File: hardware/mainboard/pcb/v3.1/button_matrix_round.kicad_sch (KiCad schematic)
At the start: 6 parts, among them U27 touch_but_round, U28 touch_but_round, U29 touch_but_round

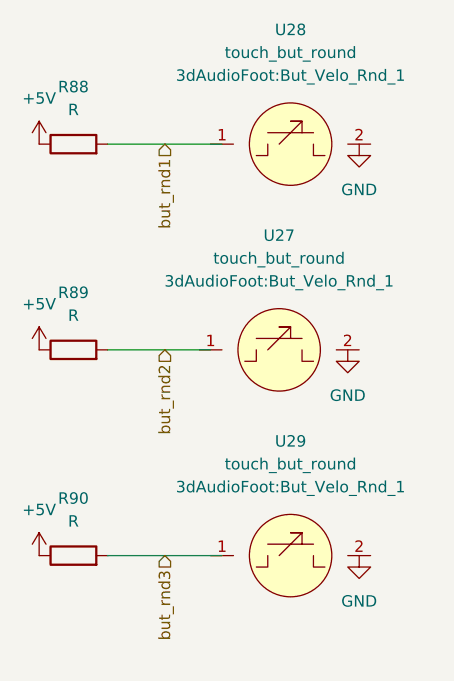
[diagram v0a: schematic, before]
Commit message: .
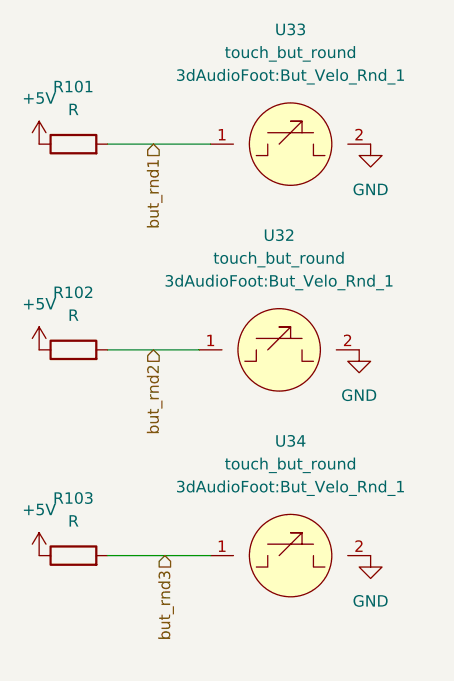
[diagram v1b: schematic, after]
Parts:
- renumbered R88 to R101, R89 to R102, R90 to R103, U27 to U32, U28 to U33, U29 to U34
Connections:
- net GND: now also U32.2, U33.2, U34.2
- net but_rnd1: now also U33.1
- net but_rnd2: now also U32.1
- net but_rnd3: now also U34.1
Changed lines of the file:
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@@
 (kicad_sch (version 20211123) (generator eeschema)
   (paper "A4")
-  (wire (pts (xy 85.09 54.61) (xy 97.79 54.61))
+  (wire (pts (xy 85.09 54.61) (xy 96.52 54.61))
     (stroke (width 0) (type default) (color 0 0 0 0))
   )
-  (wire (pts (xy 85.09 77.47) (xy 96.52 77.47))
+  (wire (pts (xy 85.09 100.33) (xy 96.52 100.33))
     (stroke (width 0) (type default) (color 0 0 0 0))
   )
-  (wire (pts (xy 85.09 100.33) (xy 97.79 100.33))
+  (wire (pts (xy 85.09 77.47) (xy 95.25 77.47))
     (stroke (width 0) (type default) (color 0 0 0 0))
   )
@@
     (effects (font (size 1.27 1.27)) (justify right))
   )
-  (hierarchical_label "but_rnd2" (shape input) (at 91.44 77.47 270)
+  (hierarchical_label "but_rnd2" (shape input) (at 90.17 77.47 270)
     (effects (font (size 1.27 1.27)) (justify right))
   )
-  (hierarchical_label "but_rnd1" (shape input) (at 91.44 54.61 270)
+  (hierarchical_label "but_rnd1" (shape input) (at 90.17 54.61 270)
     (effects (font (size 1.27 1.27)) (justify right))
   )
   (symbol (lib_id "Device:R") (at 81.28 100.33 90) (unit 1)
     (in_bom yes) (on_board yes) (fields_autoplaced)
-    (property "Reference" "R90" (id 0) (at 81.28 93.98 90))
+    (property "Reference" "R103" (id 0) (at 81.28 93.98 90))
     (property "Value" "R" (id 1) (at 81.28 96.52 90))
     (property "Footprint" "Resistor_SMD:R_1206_3216Metric_Pad1.30x1.75mm_HandSolder" (id 2) (at 81.28 102.108 90)
@@
   (symbol (lib_id "Device:R") (at 81.28 54.61 90) (unit 1)
     (in_bom yes) (on_board yes) (fields_autoplaced)
-    (property "Reference" "R88" (id 0) (at 81.28 48.26 90))
+    (property "Reference" "R101" (id 0) (at 81.28 48.26 90))
     (property "Value" "R" (id 1) (at 81.28 50.8 90))
     (property "Footprint" "Resistor_SMD:R_1206_3216Metric_Pad1.30x1.75mm_HandSolder" (id 2) (at 81.28 56.388 90)
@@
     (pin "2")
   )
-  (symbol (lib_id "power:GND") (at 111.76 77.47 0) (unit 1)
+  (symbol (lib_id "power:GND") (at 113.03 77.47 0) (unit 1)
     (in_bom yes) (on_board yes) (fields_autoplaced)
-    (property "Reference" "#PWR070" (id 0) (at 111.76 83.82 0)
+    (property "Reference" "#PWR079" (id 0) (at 113.03 83.82 0)
       (effects (font (size 1.27 1.27)) hide)
     )
-    (property "Value" "GND" (id 1) (at 111.76 82.55 0))
-    (property "Footprint" "" (id 2) (at 111.76 77.47 0)
+    (property "Value" "GND" (id 1) (at 113.03 82.55 0))
+    (property "Footprint" "" (id 2) (at 113.03 77.47 0)
       (effects (font (size 1.27 1.27)) hide)
     )
-    (property "Datasheet" "" (id 3) (at 111.76 77.47 0)
+    (property "Datasheet" "" (id 3) (at 113.03 77.47 0)
       (effects (font (size 1.27 1.27)) hide)
     )
     (pin "1")
   )
-  (symbol (lib_id "power:GND") (at 113.03 100.33 0) (unit 1)
+  (symbol (lib_id "power:GND") (at 114.3 100.33 0) (unit 1)
     (in_bom yes) (on_board yes) (fields_autoplaced)
-    (property "Reference" "#PWR072" (id 0) (at 113.03 106.68 0)
+    (property "Reference" "#PWR081" (id 0) (at 114.3 106.68 0)
       (effects (font (size 1.27 1.27)) hide)
     )
-    (property "Value" "GND" (id 1) (at 113.03 105.41 0))
-    (property "Footprint" "" (id 2) (at 113.03 100.33 0)
+    (property "Value" "GND" (id 1) (at 114.3 105.41 0))
+    (property "Footprint" "" (id 2) (at 114.3 100.33 0)
       (effects (font (size 1.27 1.27)) hide)
     )
-    (property "Datasheet" "" (id 3) (at 113.03 100.33 0)
+    (property "Datasheet" "" (id 3) (at 114.3 100.33 0)
       (effects (font (size 1.27 1.27)) hide)
     )
     (pin "1")
   )
-  (symbol (lib_id "power:GND") (at 113.03 54.61 0) (unit 1)
+  (symbol (lib_id "power:GND") (at 114.3 54.61 0) (unit 1)
     (in_bom yes) (on_board yes) (fields_autoplaced)
-    (property "Reference" "#PWR071" (id 0) (at 113.03 60.96 0)
+    (property "Reference" "#PWR080" (id 0) (at 114.3 60.96 0)
       (effects (font (size 1.27 1.27)) hide)
     )
-    (property "Value" "GND" (id 1) (at 113.03 59.69 0))
-    (property "Footprint" "" (id 2) (at 113.03 54.61 0)
+    (property "Value" "GND" (id 1) (at 114.3 59.69 0))
+    (property "Footprint" "" (id 2) (at 114.3 54.61 0)
       (effects (font (size 1.27 1.27)) hide)
     )
-    (property "Datasheet" "" (id 3) (at 113.03 54.61 0)
+    (property "Datasheet" "" (id 3) (at 114.3 54.61 0)
       (effects (font (size 1.27 1.27)) hide)
     )
@@
   (symbol (lib_id "3dAudioSym:touch_but_round") (at 105.41 101.6 0) (unit 1)
     (in_bom yes) (on_board yes) (fields_autoplaced)
-    (property "Reference" "U29" (id 0) (at 105.41 87.63 0))
+    (property "Reference" "U34" (id 0) (at 105.41 87.63 0))
     (property "Value" "touch_but_round" (id 1) (at 105.41 90.17 0))
     (property "Footprint" "3dAudioFoot:But_Velo_Rnd_1" (id 2) (at 105.41 92.71 0))
@@
   (symbol (lib_id "power:+5V") (at 77.47 100.33 0) (unit 1)
     (in_bom yes) (on_board yes) (fields_autoplaced)
-    (property "Reference" "#PWR069" (id 0) (at 77.47 104.14 0)
+    (property "Reference" "#PWR078" (id 0) (at 77.47 104.14 0)
       (effects (font (size 1.27 1.27)) hide)
     )
@@
   (symbol (lib_id "power:+5V") (at 77.47 77.47 0) (unit 1)
     (in_bom yes) (on_board yes) (fields_autoplaced)
-    (property "Reference" "#PWR068" (id 0) (at 77.47 81.28 0)
+    (property "Reference" "#PWR077" (id 0) (at 77.47 81.28 0)
       (effects (font (size 1.27 1.27)) hide)
     )
@@
   (symbol (lib_name "touch_but_round_1") (lib_id "3dAudioSym:touch_but_round") (at 105.41 55.88 0) (unit 1)
     (in_bom yes) (on_board yes) (fields_autoplaced)
-    (property "Reference" "U28" (id 0) (at 105.41 41.91 0))
+    (property "Reference" "U33" (id 0) (at 105.41 41.91 0))
     (property "Value" "touch_but_round" (id 1) (at 105.41 44.45 0))
     (property "Footprint" "3dAudioFoot:But_Velo_Rnd_1" (id 2) (at 105.41 46.99 0))
@@
   (symbol (lib_id "power:+5V") (at 77.47 54.61 0) (unit 1)
     (in_bom yes) (on_board yes) (fields_autoplaced)
-    (property "Reference" "#PWR067" (id 0) (at 77.47 58.42 0)
+    (property "Reference" "#PWR076" (id 0) (at 77.47 58.42 0)
       (effects (font (size 1.27 1.27)) hide)
     )
@@
   (symbol (lib_id "Device:R") (at 81.28 77.47 90) (unit 1)
     (in_bom yes) (on_board yes) (fields_autoplaced)
-    (property "Reference" "R89" (id 0) (at 81.28 71.12 90))
+    (property "Reference" "R102" (id 0) (at 81.28 71.12 90))
     (property "Value" "R" (id 1) (at 81.28 73.66 90))
     (property "Footprint" "Resistor_SMD:R_1206_3216Metric_Pad1.30x1.75mm_HandSolder" (id 2) (at 81.28 79.248 90)
@@
   (symbol (lib_name "touch_but_round_2") (lib_id "3dAudioSym:touch_but_round") (at 104.14 78.74 0) (unit 1)
     (in_bom yes) (on_board yes) (fields_autoplaced)
-    (property "Reference" "U27" (id 0) (at 104.14 64.77 0))
+    (property "Reference" "U32" (id 0) (at 104.14 64.77 0))
     (property "Value" "touch_but_round" (id 1) (at 104.14 67.31 0))
     (property "Footprint" "3dAudioFoot:But_Velo_Rnd_1" (id 2) (at 104.14 69.85 0))
